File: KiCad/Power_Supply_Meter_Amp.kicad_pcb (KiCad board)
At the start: 4 copper layers, 150 x 85.2 mm, 84 parts, among them J10 VCC_IN, J11 VCC_OUT, J13 EMK_Out, J14 EMK_Out, J21 Conn_01x05_bridged, J30 Pegel_In, J31 Pegel_In, J32 Pegel_In, J33 Pegel_In, J34 LED_Out, J36 VU_Meter_Out, SW1 SW_DPST, SW9 SW_Rotary_1x4, U23 TL074, U24 TL074, U6 REC10K-2409, U7 REC10K-2415

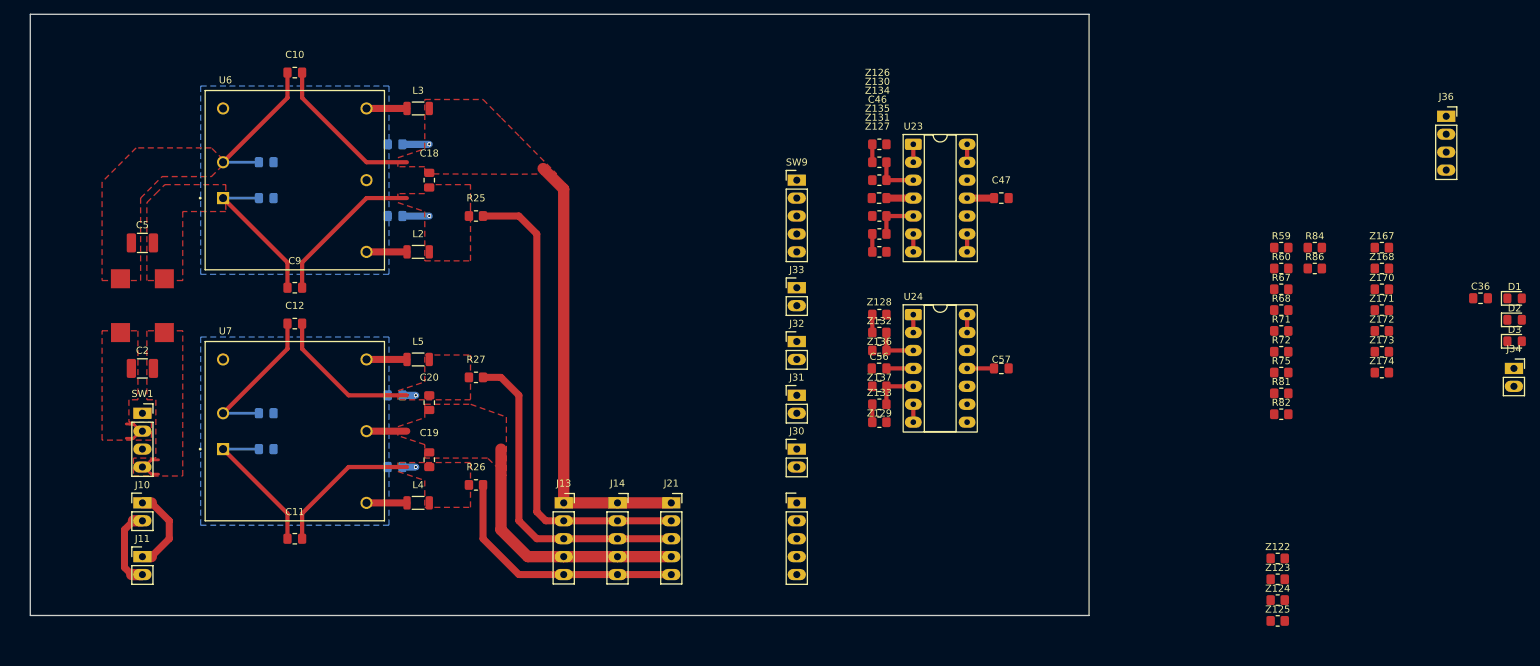
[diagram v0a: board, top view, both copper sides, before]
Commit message: PCB Update
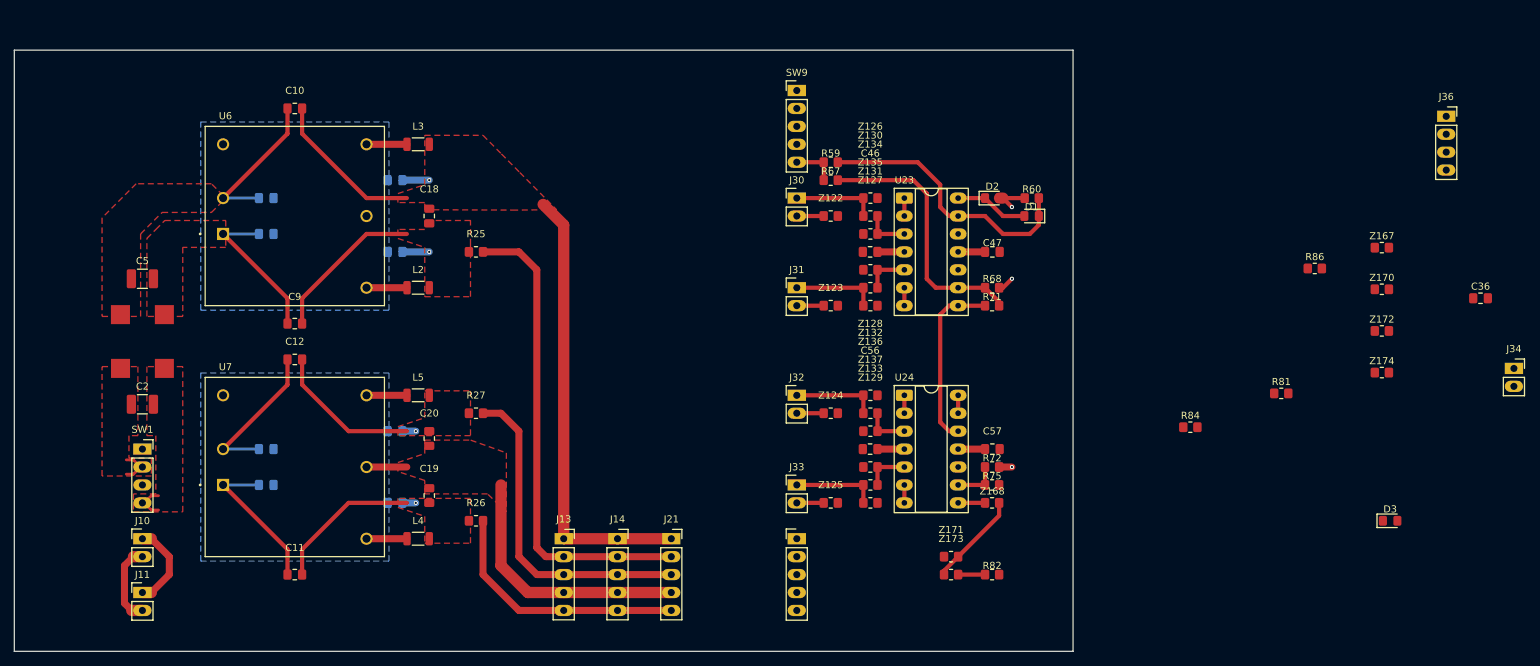
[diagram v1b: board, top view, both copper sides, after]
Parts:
- moved Z122 79.8 mm to (153.4, 68.6)
- moved D2 76.0 mm to (176.3, 66.0)
- moved Z123 74.2 mm to (153.4, 81.3)
- moved Z171 70.3 mm to (170.4, 116.8), turned to 180 degrees
- moved D1 69.4 mm to (181.9, 68.6), turned to 180 degrees
- moved Z173 68.7 mm to (170.4, 119.4)
- moved Z124 68.6 mm to (153.4, 96.5)
- moved R67 65.7 mm to (153.4, 63.5)
- moved Z125 65.5 mm to (153.4, 109.2)
- moved R59 65.0 mm to (153.4, 61.0)
- moved Z168 64.4 mm to (176.3, 109.2)
- moved R82 46.8 mm to (176.3, 119.4), turned to 180 degrees
- moved R72 44.1 mm to (176.3, 104.1), turned to 180 degrees
- moved R75 44.0 mm to (176.3, 106.7), turned to 180 degrees
- moved R71 41.1 mm to (176.3, 81.3), turned to 180 degrees
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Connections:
- R67 pad 2: Net-(U23D--) -> Net-(U23C--)
- R68 pad 2: Net-(U23D--) -> Net-(U23C--)
- R71 pad 1: Net-(U23D--) -> Net-(U23C--)
- R72 pad 1: +15V -> +15V_M
- SW9 pad 1: /Pegel_Pre -> /Pegel_Post
- SW9 pad 2: /Pegel_Mic_Effekt -> /Pegel_Aux_Return
- SW9 pad 3: /Pegel_Aux_Return -> /Pegel_Mic_Effekt
- SW9 pad 4: /Pegel_Post -> /Pegel_Pre
- U23 pad 13: Net-(U23D--) -> Net-(D1-K)
- U23 pad 14: Net-(U24C-+) -> Net-(D1-A)
- U23 pad 8: Net-(D1-A) -> Net-(U24C-+)
- U23 pad 9: Net-(D1-K) -> Net-(U23C--)
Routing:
- net +15V_M: track 7.62 -> 124.0 mm, vias 0 -> 1
- net -15V_M: track 7.62 -> 110.5 mm
- net /Pegel_Post: track 2.54 -> 80.1 mm
- net /Pegel_Aux_Return: track 5.08 -> 63.1 mm
- net /Pegel_Mic_Effekt: track 2.54 -> 42.7 mm
- net Net-(D1-K): track 0.00 -> 38.1 mm
- net Net-(U23C--): track 0.00 -> 37.6 mm
- net Net-(U24C-+): track 2.54 -> 25.2 mm
- net /Pegel_Pre: track 2.54 -> 23.9 mm
- net Net-(D2-A): track 0.00 -> 17.9 mm, vias 0 -> 2
- net Net-(Z168-Pad2): track 0.00 -> 13.4 mm
- net Net-(D1-A): track 0.00 -> 9.63 mm
- net Net-(J31-Pin_1): track 2.54 -> 12.0 mm
- net Net-(J30-Pin_1): track 2.54 -> 12.0 mm
- net Net-(J33-Pin_1): track 2.54 -> 12.0 mm
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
